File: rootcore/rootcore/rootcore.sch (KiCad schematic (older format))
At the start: 20 parts, among them J1 Conn_02x20_Odd_Even, J2 Conn_02x20_Odd_Even, J3 Conn_02x08_Odd_Even, J4 Conn_01x04_Male, J5 Conn_01x02_Male, U1 STM32F373RCTx, U2 LM13700, U3 AP1117-15, U4 LM4040DCK-2.5, Y1 Crystal

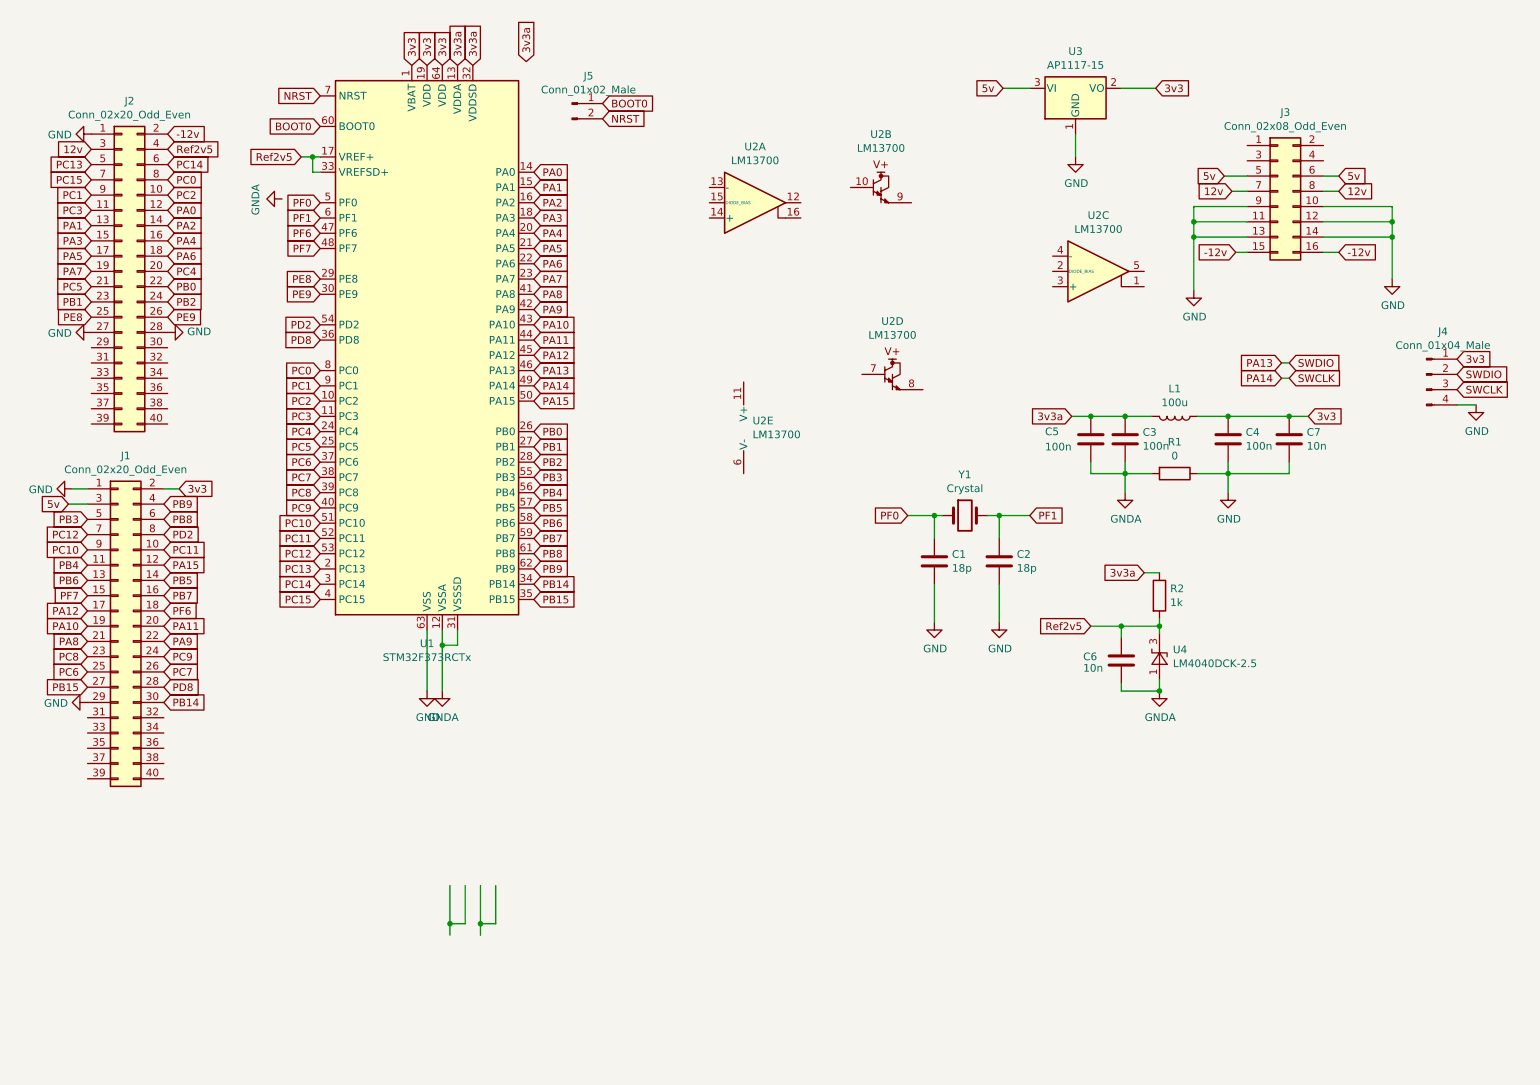
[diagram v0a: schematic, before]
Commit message: base layoyut done
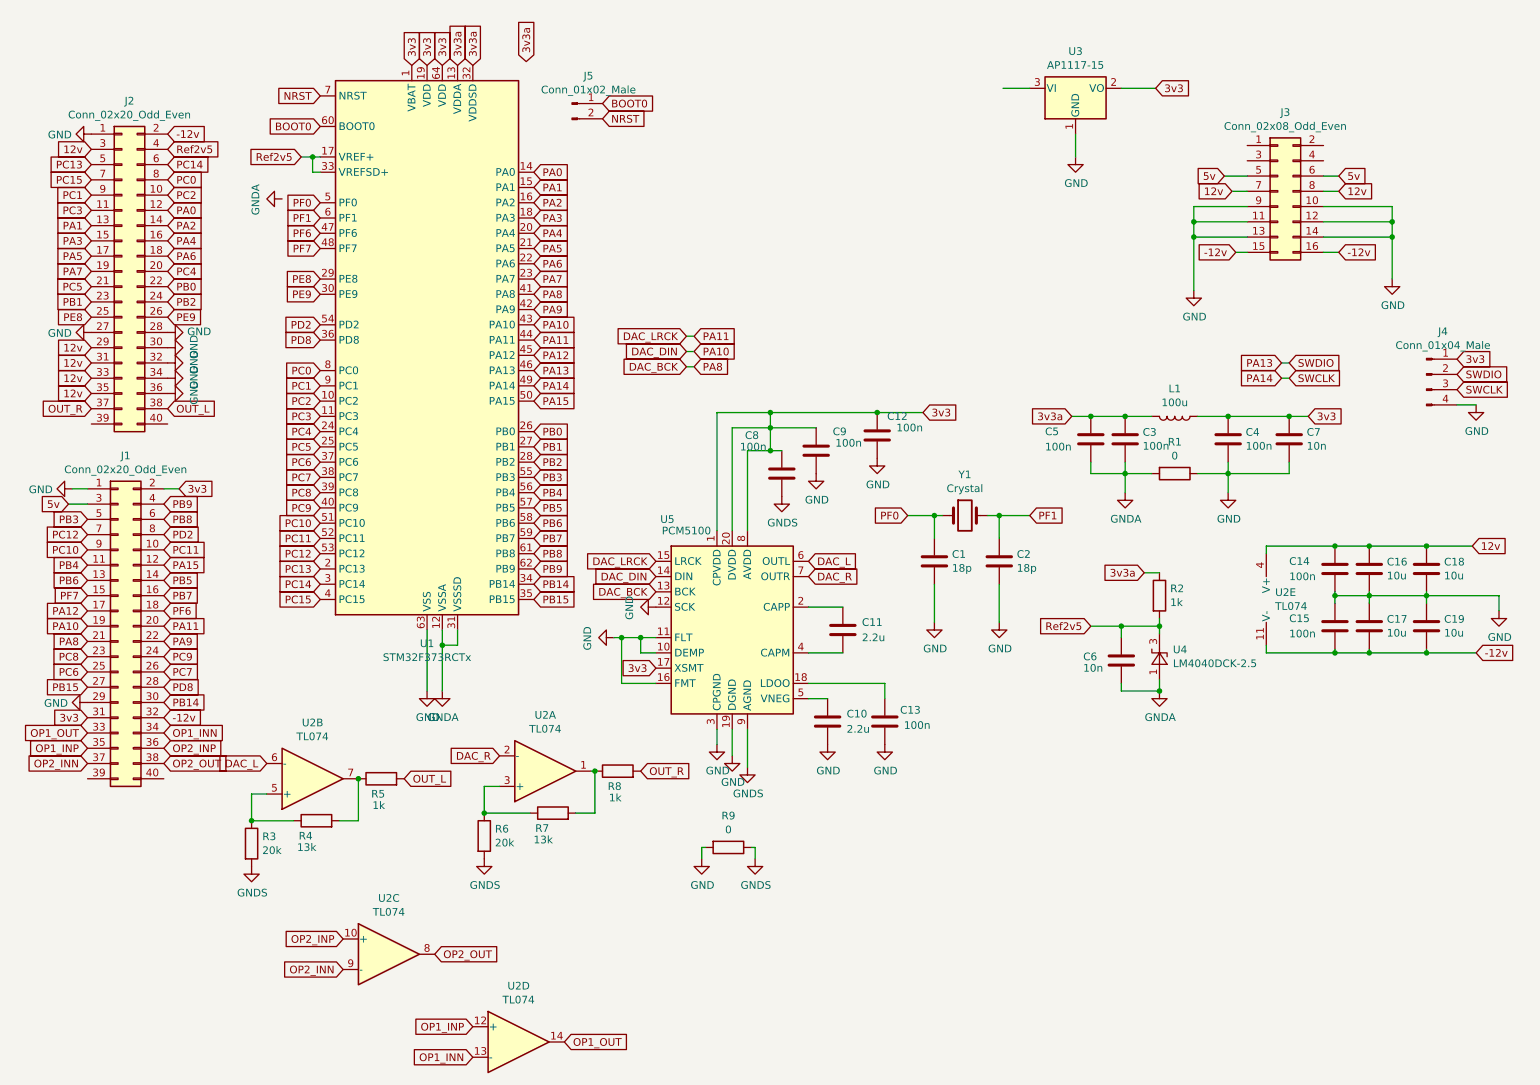
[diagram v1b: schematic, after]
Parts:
- removed U2: LM13700, Package_SO:SOIC-16_3.9x9.9mm_P1.27mm, symbol Amplifier_Operational:LM13700
- added C10, C11: 2.2u, Capacitor_SMD:C_0805_2012Metric_Pad1.18x1.45mm_HandSolder, symbol Device:C
- added C12, C13, C14, C15, C8, C9: 100n, Capacitor_SMD:C_0805_2012Metric_Pad1.18x1.45mm_HandSolder, symbol Device:C
- added C16, C17, C18, C19: 10u, Capacitor_SMD:C_0805_2012Metric_Pad1.18x1.45mm_HandSolder, symbol Device:C
- added R3, R6: 20k, Resistor_SMD:R_0805_2012Metric_Pad1.20x1.40mm_HandSolder, symbol Device:R
- added R4, R7: 13k, Resistor_SMD:R_0805_2012Metric_Pad1.20x1.40mm_HandSolder, symbol Device:R
- added R5, R8: 1k, Resistor_SMD:R_0805_2012Metric_Pad1.20x1.40mm_HandSolder, symbol Device:R
- added R9: 0, NetTie:NetTie-2_SMD_Pad0.5mm, symbol Device:R
- added U2: TL074, Package_SO:SOIC-14_3.9x8.7mm_P1.27mm, symbol Amplifier_Operational:TL074
- added U5: PCM5100, Package_SO:TSSOP-20_4.4x6.5mm_P0.65mm, symbol Audio:PCM5100
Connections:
- net labels added: DAC_BCK, DAC_DIN, DAC_L, DAC_LRCK, DAC_R, GNDS, OP1_INN, OP1_INP, OP1_OUT, OP2_INN, OP2_INP, OP2_OUT, OUT_L, OUT_R
- wire segments 77 -> 137
